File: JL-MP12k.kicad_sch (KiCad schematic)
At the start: 27 parts, among them SW1 RotaryEncoder_Switch, U1 SSD1107

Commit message: Add production files and update PCB settings
Added new production outputs including BOM, designators, netlist, and positions CSVs, as well as backup and schematic/assembly images. Updated KiCad project files to adjust drill shape, output directories, solder mask clearance, and BOM visibility. Removed obsolete CleanShot images and set several schematic components to not be included in BOM.
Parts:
- Gemini1, SW1, U1: now left out of the parts list
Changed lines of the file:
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@@
 		(unit 1)
 		(exclude_from_sim no)
-		(in_bom yes)
+		(in_bom no)
 		(on_board yes)
 		(dnp no)
@@
 		(unit 1)
 		(exclude_from_sim no)
-		(in_bom yes)
+		(in_bom no)
 		(on_board yes)
 		(dnp no)
@@
 		(unit 1)
 		(exclude_from_sim no)
-		(in_bom yes)
+		(in_bom no)
 		(on_board yes)
 		(dnp no)

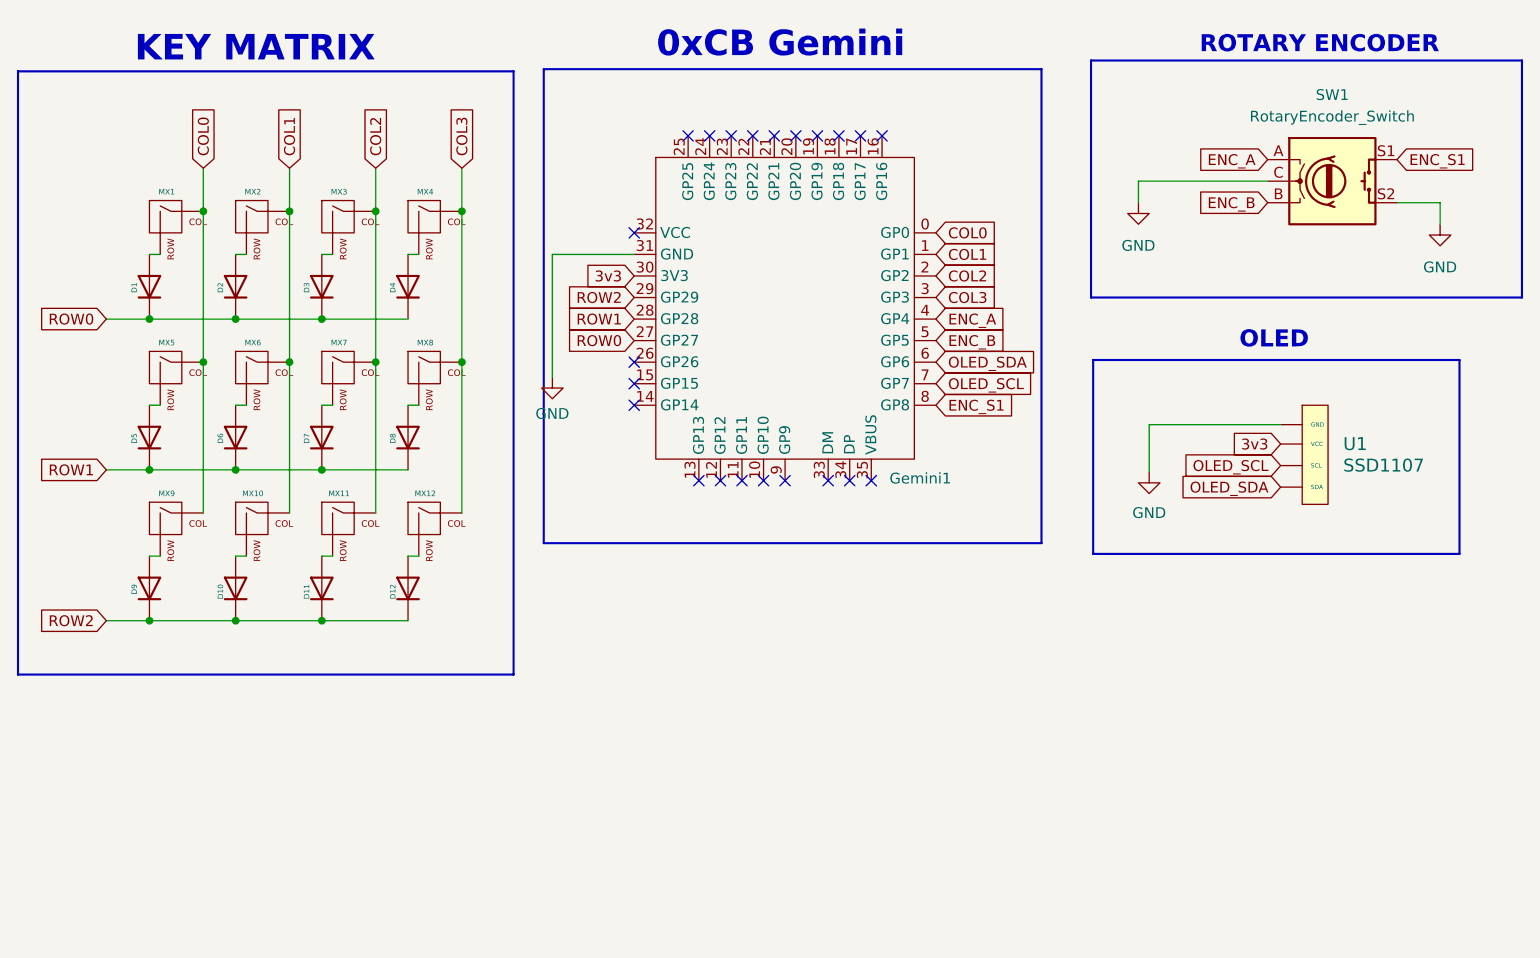
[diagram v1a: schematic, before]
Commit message: fixed some stuff
rev 1.1
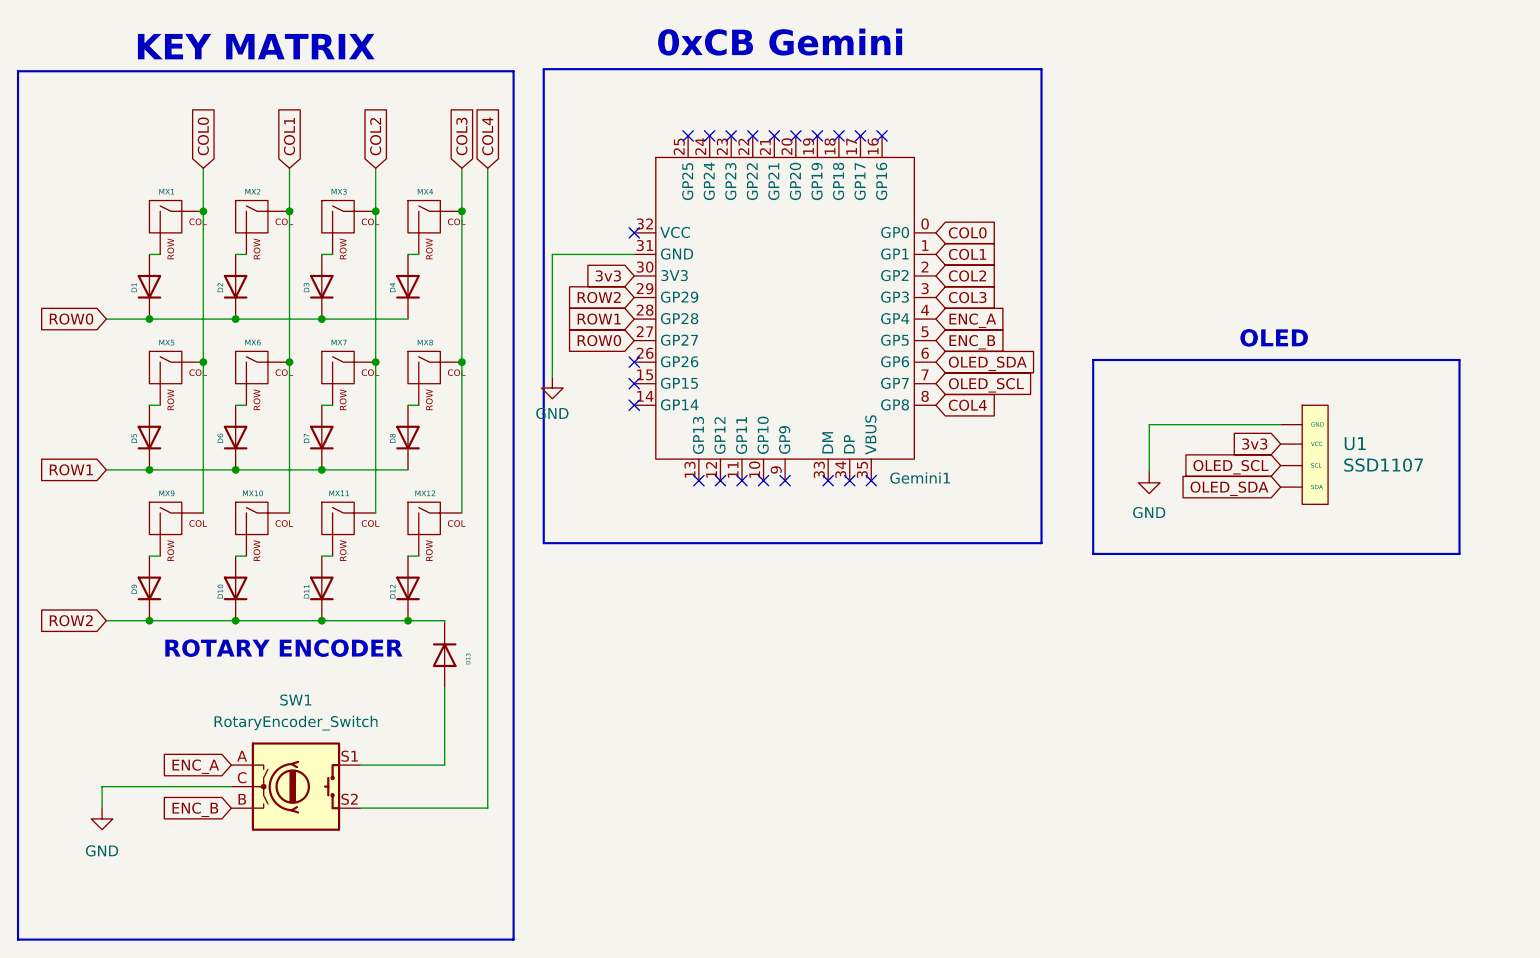
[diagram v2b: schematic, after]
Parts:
- added D13: 1N4148W, Diode_SMD:D_SOD-123, symbol Diode:1N4148W
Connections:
- net GND: no longer SW1.S2
- net ROW2: now also D13.1 (K)
- net ENC_S1: no longer names the net of SW1.S1
- net ENC_S1: now also D13.2 (A); no longer Gemini1.8 (GP8)
- new net COL4: Gemini1.8 (GP8), SW1.S2
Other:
- moved on the sheet: SW1
